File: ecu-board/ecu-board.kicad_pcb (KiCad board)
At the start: 2 copper layers, 150 x 100 mm, 49 parts, among them J1 MicroSquirt_connector, J10 Injector connector, J11 Cockpit connector, J12 EGO connector, J13 Chrankshaft Hall connector, J14 Camshaft Hall connector, J15 Ignition 1 connector, J16 Ignition 2 connector, J17 Camera connector, J18 Wheel Hall connector, J2 Battery power conenctor, J4 Motor connector, J5 Serial DB9 connector, J6 Controller connector, J7 Backlight connector, J8 IAT connector, J9 CLT connector, K1 Main power relay, K2 Start motor relay, Q1 IPD90P03P4-04, U1 MAP Sensor

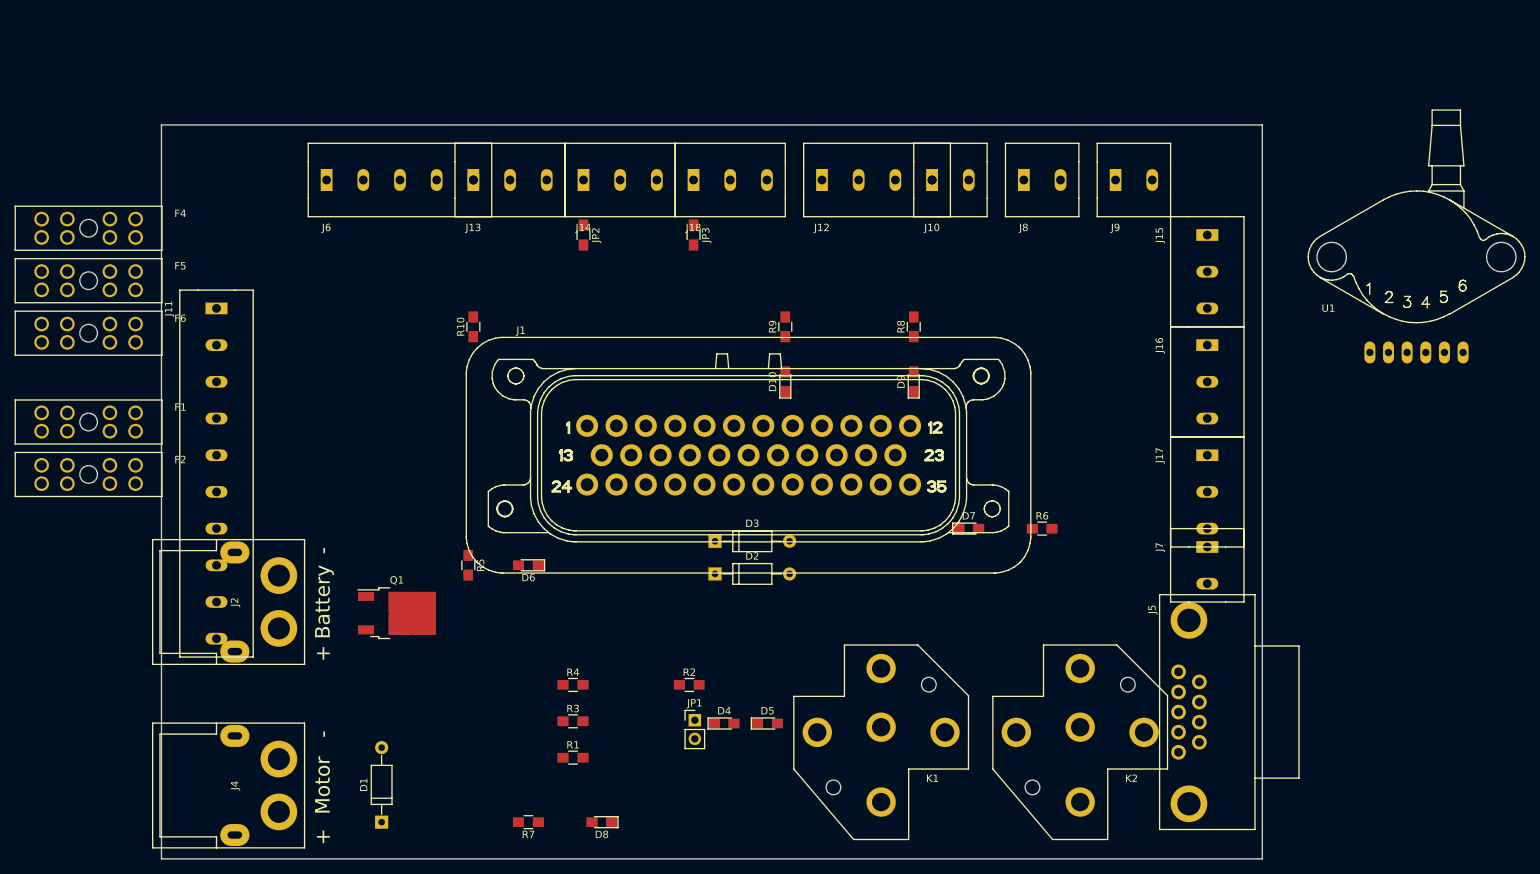
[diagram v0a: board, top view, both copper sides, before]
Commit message: Layout fuses.
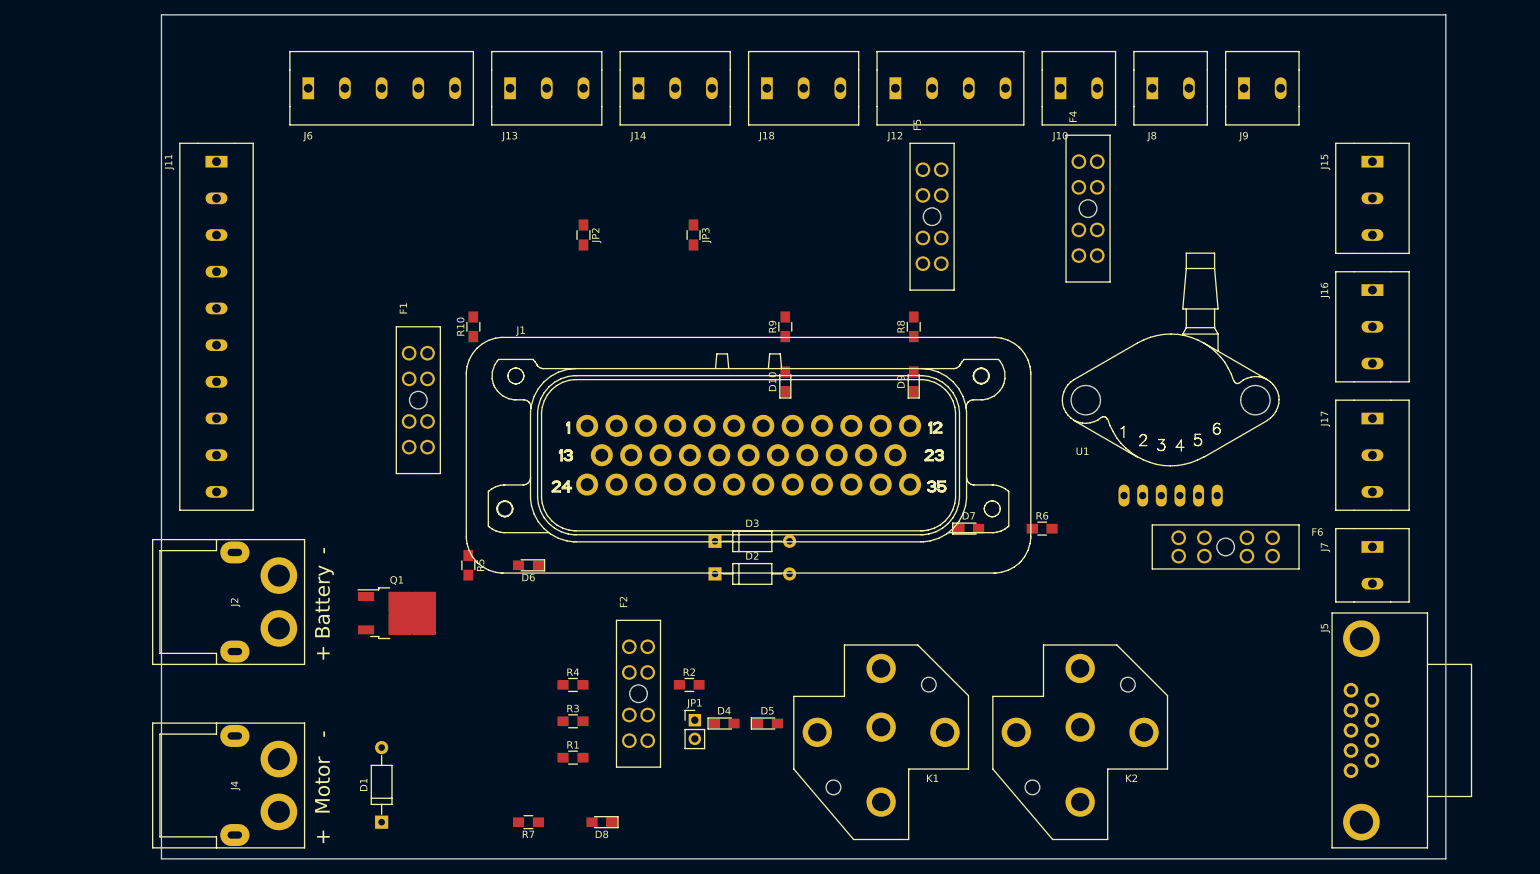
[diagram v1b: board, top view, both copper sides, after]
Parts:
- moved F6 157.6 mm to (195.0, 107.5)
- moved F4 136.2 mm to (176.2, 61.4), turned to 90 degrees
- moved F5 115.3 mm to (155.0, 62.5), turned to 90 degrees
- moved F2 80.7 mm to (115.0, 127.5), turned to 90 degrees
- moved F1 45.0 mm to (85.0, 87.5), turned to 90 degrees
- moved U1 38.8 mm to (187.5, 87.5)
- moved J15 24.6 mm to (215.0, 55.0)
- moved J16 23.7 mm to (215.0, 72.5)
- moved J5 23.6 mm to (213.5, 132.5)
- moved J17 23.0 mm to (215.0, 90.0)
- moved J7 22.5 mm to (215.0, 107.5)
- moved J10 21.5 mm to (172.5, 45.0)
- moved J8 21.5 mm to (185.0, 45.0)
- moved J9 21.5 mm to (197.5, 45.0)
- moved J11 20.0 mm to (57.5, 55.0)
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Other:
- board size 150 x 100 mm -> 175 x 115 mm
